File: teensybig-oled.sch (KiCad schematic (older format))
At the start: 3 parts, among them J1 TEENSY-LC, J2 OLED-I2C

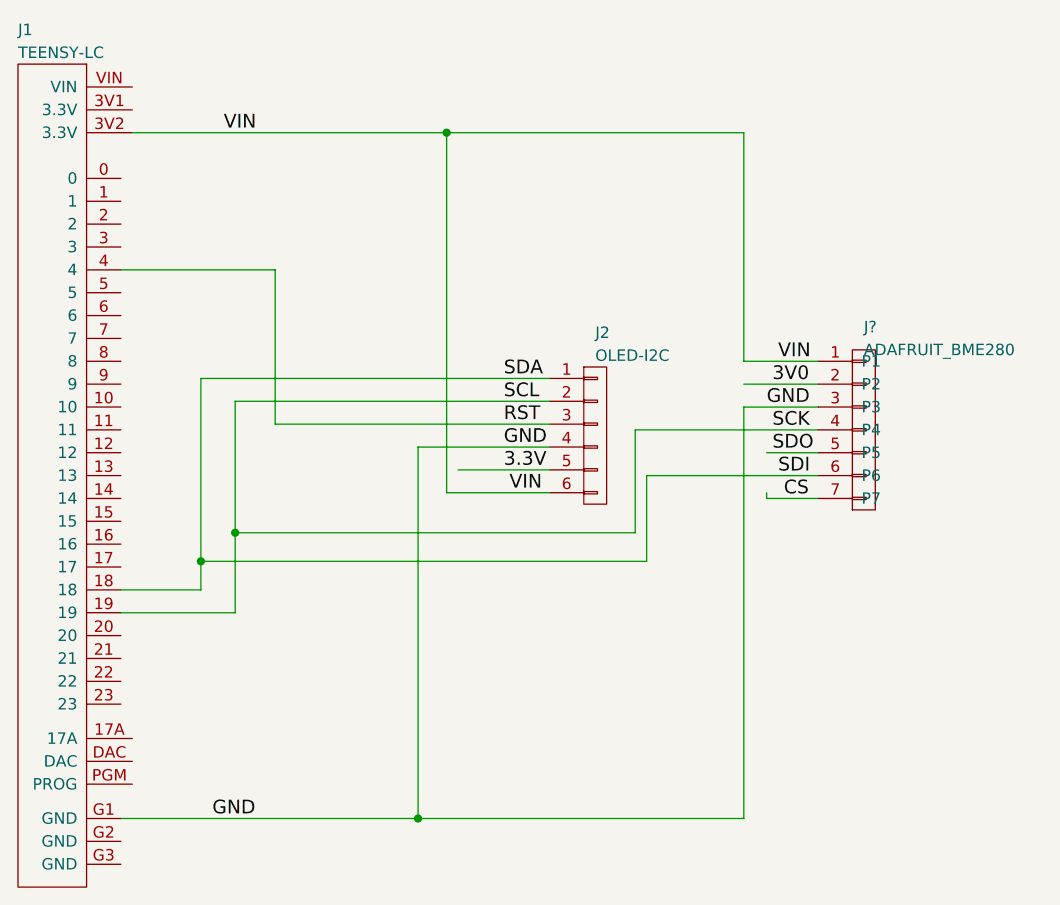
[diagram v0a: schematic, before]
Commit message: uploaded to oshpark
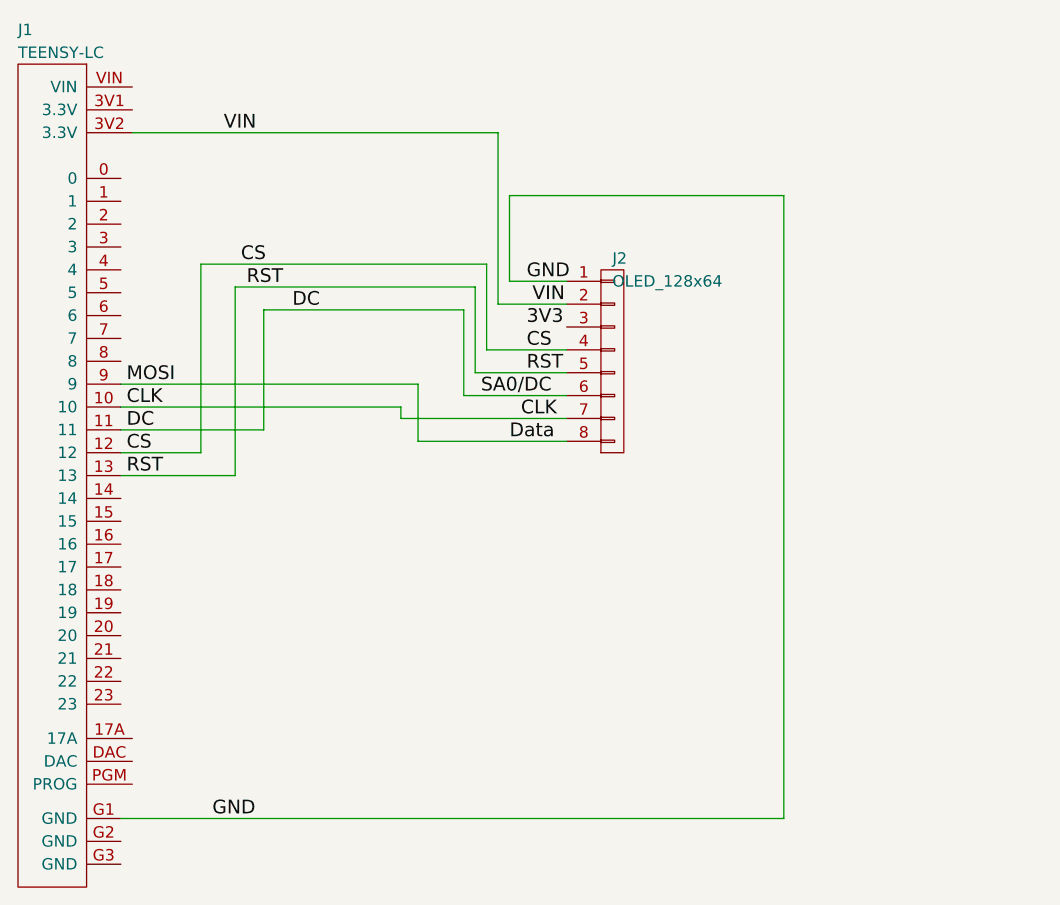
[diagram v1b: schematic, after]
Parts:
- removed J2: OLED-I2C, Wickerlib:Pin_Header_Straight_1x06, symbol HEADER-FEMALE-6POS-TH-1x06-P0.1IN
- removed J?: ADAFRUIT_BME280, CONN-1x07-2.54MM-TH, symbol HEADER-FEMALE-7POS-TH-1x07-P0.1IN
- added J2: OLED_128x64, Wickerlib:Pin_Header_Straight_1x08, symbol HEADER-FEMALE-8POS-TH-1x08-P0.1IN
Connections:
- net labels added: 3V3, CLK, DC, Data, MOSI, SA0/DC
- net labels removed: 3.3V, 3V0, SCK, SCL, SDA, SDI, SDO
- wire segments 30 -> 29
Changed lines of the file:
@@
 LIBS:valves
 LIBS:wickerlib
-LIBS:teensyi2c-cache
+LIBS:teensybig-oled-cache
 EELAYER 25 0
 EELAYER END
@@
 	1    0    0    -1
 $EndComp
+Text Label 6000 2725 0    60   ~ 0
+CS
+Text Label 6025 2825 0    60   ~ 0
+RST
+Text Label 6225 2925 0    60   ~ 0
+DC
+Text Label 5500 3350 0    60   ~ 0
+CLK
+Text Label 5500 3250 0    60   ~ 0
+MOSI
 Text Label 5925 2150 0    60   ~ 0
 VIN
 $Comp
-L HEADER-FEMALE-6POS-TH-1x06-P0.1IN J2
-U 1 1 57712F77
-P 7550 3475
-F 0 "J2" H 7550 3925 50  0000 L CNN
-F 1 "OLED-I2C" H 7550 3825 50  0000 L CNN
-F 2 "Wickerlib:Pin_Header_Straight_1x06" H 7550 3125 50  0001 C CIN
-F 3 "https://cdn.harwin.com/pdfs/60page140.pdf" H 7550 3475 5   0001 C CNN
-F 4 "Pin_Header_Straight_1x06" H 7550 3125 50  0001 C CIN "Package"
-F 5 "Harwin" H 7550 3125 50  0001 C CIN "MF_Name"
-F 6 "M20-7820642" H 7550 3125 50  0001 C CIN "MF_PN"
-F 7 "Digikey" H 7550 3125 50  0001 C CIN "S1_Name"
-F 8 "952-1808-ND" H 7550 3125 50  0001 C CIN "S1_PN"
-F 9 "HEADER FEMALE 6POS TH 1x06 0.1”" H 7550 3125 50  0001 C CIN "Description"
-F 10 "Not Verified" H 7550 3125 50  0001 C CIN "Verified"
-	1    7550 3475
+L HEADER-FEMALE-8POS-TH-1x08-P0.1IN J2
+U 1 1 573AD5FE
+P 7625 3150
+F 0 "J2" H 7625 3600 50  0000 L CNN
+F 1 "OLED_128x64" H 7625 3500 50  0000 L CNN
+F 2 "Wickerlib:Pin_Header_Straight_1x08" H 7625 2800 50  0001 C CIN
+F 3 "https://cdn.harwin.com/pdfs/60page140.pdf" H 7625 3150 5   0001 C CNN
+F 4 "Pin_Header_Straight_1x08" H 7625 2800 50  0001 C CIN "Package"
+F 5 "Harwin" H 7625 2800 50  0001 C CIN "MF_Name"
+F 6 "M20-7820842" H 7625 2800 50  0001 C CIN "MF_PN"
+F 7 "Digikey" H 7625 2800 50  0001 C CIN "S1_Name"
+F 8 "952-1823-ND" H 7625 2800 50  0001 C CIN "S1_PN"
+F 9 "HEADER FEMALE 8POS TH 1x08 0.1”" H 7625 2800 50  0001 C CIN "Description"
+F 10 "Not Verified" H 7625 2800 50  0001 C CIN "Verified"
+	1    7625 3150
 	1    0    0    -1
 $EndComp
-Wire Wire Line
-	5525 2150 8200 2150
-Wire Wire Line
-	5825 3225 7350 3225
-Wire Wire Line
-	5975 3325 7350 3325
-Wire Wire Line
-	6150 3425 7350 3425
-Wire Wire Line
-	6775 3525 7350 3525
-Wire Wire Line
-	7350 3625 6950 3625
-Wire Wire Line
-	7350 3725 6900 3725
-Text Label 7150 3225 0    60   ~ 0
-SDA
-Text Label 7150 3325 0    60   ~ 0
-SCL
-Text Label 7150 3425 0    60   ~ 0
+Text Label 7250 2800 0    60   ~ 0
+GND
+Text Label 7275 2900 0    60   ~ 0
+VIN
+Text Label 7250 3000 0    60   ~ 0
+3V3
+Text Label 7250 3100 0    60   ~ 0
+CS
+Text Label 7250 3200 0    60   ~ 0
 RST
-Text Label 7150 3525 0    60   ~ 0
-GND
-Text Label 7150 3625 0    60   ~ 0
-3.3V
-Text Label 7175 3725 0    60   ~ 0
-VIN
-Wire Wire Line
-	5825 3225 5825 4150
-Wire Wire Line
-	5825 4150 5475 4150
-Wire Wire Line
-	5975 3325 5975 4250
-Wire Wire Line
-	5975 4250 5475 4250
-Wire Wire Line
-	6150 3425 6150 2750
-Wire Wire Line
-	6150 2750 5475 2750
-Wire Wire Line
-	6775 3525 6775 5150
+Text Label 7050 3300 0    60   ~ 0
+SA0/DC
+Text Label 7225 3400 0    60   ~ 0
+CLK
+Text Label 7175 3500 0    60   ~ 0
+Data
 Text Label 5875 5150 0    60   ~ 0
 GND
+Text Label 5500 3550 0    60   ~ 0
+CS
+Text Label 5500 3650 0    60   ~ 0
+RST
+Text Label 5500 3450 0    60   ~ 0
+DC
 Wire Wire Line
-	5475 5150 8200 5150
+	5825 2725 7075 2725
 Wire Wire Line
-	6900 3725 6900 2150
-$Comp
-L HEADER-FEMALE-7POS-TH-1x07-P0.1IN J?
-U 1 1 57713409
-P 8725 3450
-F 0 "J?" H 8725 3900 50  0000 L CNN
-F 1 "ADAFRUIT_BME280" H 8725 3800 50  0000 L CNN
-F 2 "CONN-1x07-2.54MM-TH" H 8725 3100 50  0001 C CIN
-F 3 "https://cdn.harwin.com/pdfs/60page140.pdf" H 8725 3450 5   0001 C CNN
-F 4 "Pin_Header_Straight_1x07" H 8725 3100 50  0001 C CIN "Package"
-F 5 "Harwin" H 8725 3100 50  0001 C CIN "MF_Name"
-F 6 "M20-7822046" H 8725 3100 50  0001 C CIN "MF_PN"
-F 7 "Digikey" H 8725 3100 50  0001 C CIN "S1_Name"
-F 8 "952-1905-ND" H 8725 3100 50  0001 C CIN "S1_PN"
-F 9 "HEADER FEMALE 7POS TH 1x07 0.1”" H 8725 3100 50  0001 C CIN "Description"
-F 10 "Not Verified" H 8725 3100 50  0001 C CIN "Verified"
-	1    8725 3450
-	1    0    0    -1
-$EndComp
+	5825 2725 5825 3550
 Wire Wire Line
-	8525 3150 8200 3150
+	5825 3550 5475 3550
 Wire Wire Line
-	8200 3150 8200 2150
-Connection ~ 6900 2150
+	5975 2825 5975 3650
 Wire Wire Line
-	8525 3350 8200 3350
+	5975 3650 5475 3650
 Wire Wire Line
-	8200 3350 8200 5150
-Connection ~ 6775 5150
+	5475 3450 6100 3450
 Wire Wire Line
-	8525 3450 7725 3450
+	6100 3450 6100 2925
 Wire Wire Line
-	7725 3450 7725 3900
+	5475 3350 6700 3350
 Wire Wire Line
-	7725 3900 5975 3900
-Connection ~ 5975 3900
+	5475 3250 6775 3250
 Wire Wire Line
-	8525 3650 7775 3650
+	5525 2150 7125 2150
 Wire Wire Line
-	7775 3650 7775 4025
+	6700 3400 7425 3400
 Wire Wire Line
-	7775 4025 5825 4025
-Connection ~ 5825 4025
+	6975 2925 6975 3300
 Wire Wire Line
-	8525 3250 8200 3250
+	6100 2925 6975 2925
 Wire Wire Line
-	8300 3550 8525 3550
+	6775 3500 7425 3500
 Wire Wire Line
-	8525 3750 8300 3750
+	5475 5150 8375 5150
 Wire Wire Line
-	8300 3750 8300 3725
-Text Label 8350 3150 0    60   ~ 0
-VIN
-Text Label 8325 3250 0    60   ~ 0
-3V0
-Text Label 8300 3350 0    60   ~ 0
-GND
-Text Label 8325 3450 0    60   ~ 0
-SCK
-Text Label 8325 3550 0    60   ~ 0
-SDO
-Text Label 8350 3650 0    60   ~ 0
-SDI
-Text Label 8375 3750 0    60   ~ 0
-CS
+	8375 5150 8375 2425
+Wire Wire Line
+	8375 2425 7175 2425
+Wire Wire Line
+	7175 2425 7175 2800
+Wire Wire Line
+	7175 2800 7425 2800
+Wire Wire Line
+	7425 2900 7125 2900
+Wire Wire Line
+	7125 2900 7125 2150
+Wire Wire Line
+	7075 2725 7075 3100
+Wire Wire Line
+	7075 3100 7425 3100
+Wire Wire Line
+	6975 3300 7425 3300
+Wire Wire Line
+	7025 2825 7025 3200
+Wire Wire Line
+	7025 3200 7425 3200
+Wire Wire Line
+	6700 3350 6700 3400
+Wire Wire Line
+	5975 2825 7025 2825
+Wire Wire Line
+	6775 3250 6775 3500
 $EndSCHEMATC
